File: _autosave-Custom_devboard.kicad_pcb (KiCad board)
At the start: 2 copper layers, 21 x 51 mm, 32 parts, among them J1 USB_C_Receptacle_USB2.0_14P, J2 Conn_01x20, J3 Conn_01x20, J4 Conn_01x03, SW1 SW_Push, U1 RP2040, U2 MCP1700x-330xxTT, U4 W25Q16JVZPIQ TR, Y1 12 MHz

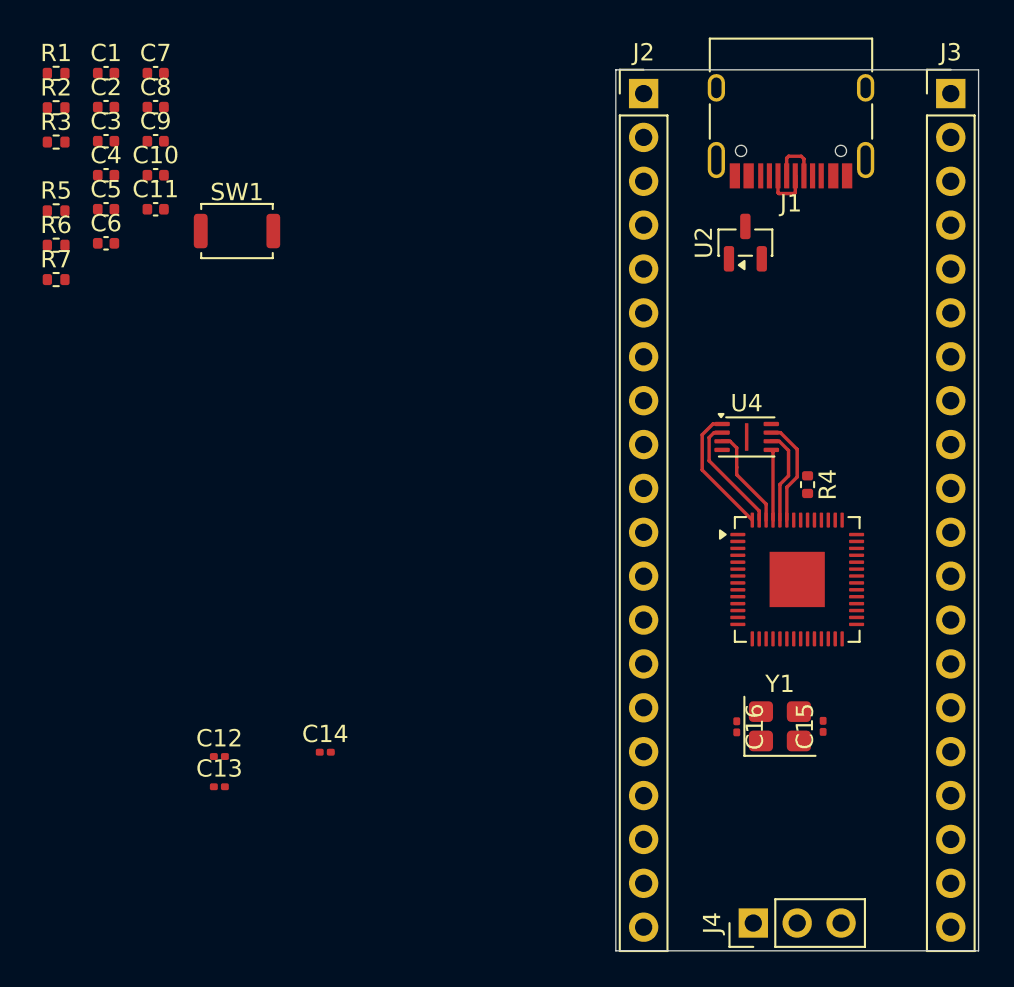
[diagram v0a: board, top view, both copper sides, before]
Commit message: PCB, CONECTING EVERYHTING SUCKS SO BAD
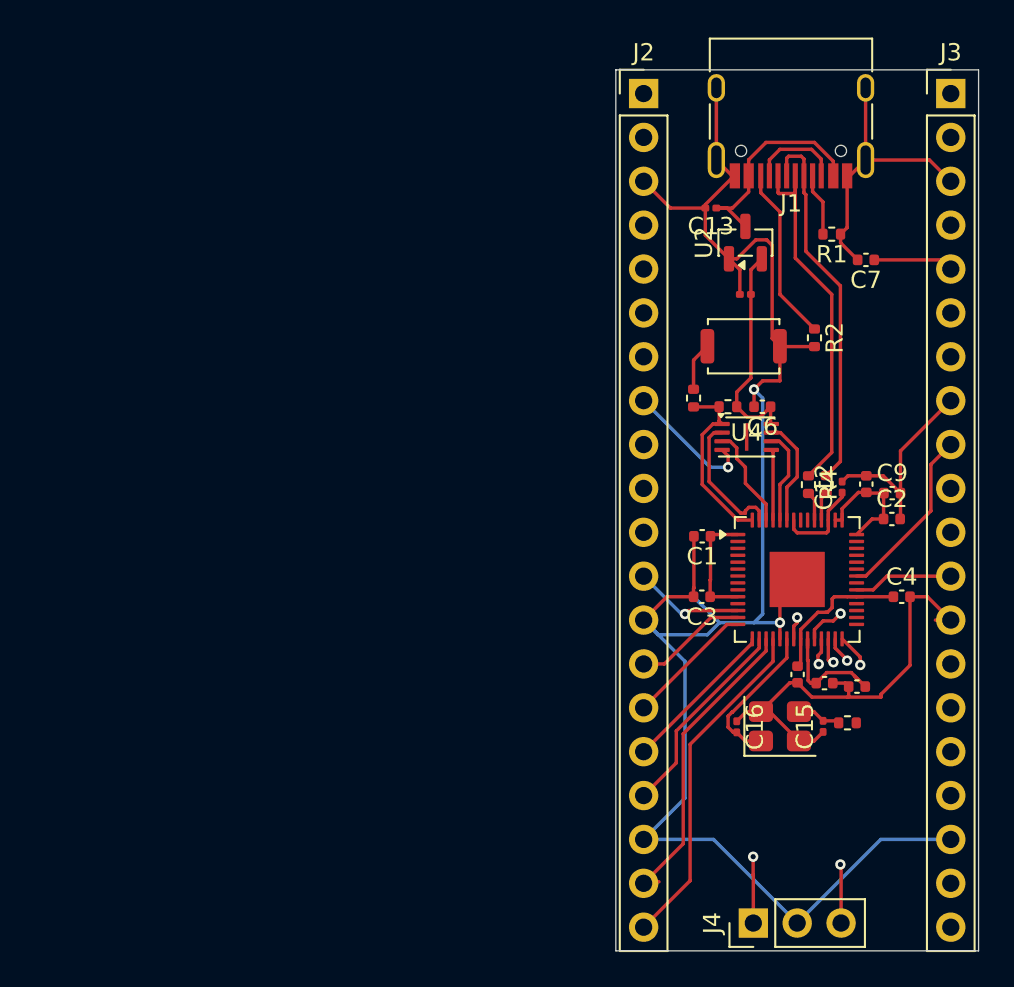
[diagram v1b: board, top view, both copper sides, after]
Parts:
- moved R5 54.6 mm to (216.4, 111.3)
- moved C4 52.1 mm to (219.6, 104.0)
- moved C2 51.4 mm to (219.0, 99.5)
- moved C10 50.2 mm to (217.0, 109.2), turned to 180 degrees
- moved R3 48.8 mm to (215.2, 97.5), turned to -90 degrees
- moved C5 48.2 mm to (213.5, 108.5), turned to -90 degrees
- moved C11 47.5 mm to (215.1, 109.0)
- moved C9 47.3 mm to (219.0, 98.0)
- moved C8 46.6 mm to (217.5, 97.5), turned to 90 degrees
- moved R2 45.9 mm to (214.5, 89.0), turned to -90 degrees
- moved R1 45.9 mm to (215.5, 83.0), turned to 180 degrees
- moved C13 44.0 mm to (208.5, 81.5), turned to 180 degrees
- moved C1 43.7 mm to (208.0, 100.5), turned to 180 degrees
- moved C3 43.4 mm to (208.0, 104.0), turned to 180 degrees
- moved C7 42.5 mm to (217.5, 84.5), turned to 180 degrees
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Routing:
- net GND: track 0.00 -> 169.0 mm, vias 0 -> 3
- net +3V3: track 0.00 -> 40.0 mm
- net GPIO15: track 0.00 -> 19.8 mm
- net USBD+: track 2.99 -> 21.8 mm
- net USBD-: track 3.11 -> 21.7 mm
- net GPIO14: track 0.00 -> 18.0 mm
- net VBUS: track 0.00 -> 13.0 mm
- net +1V1: track 0.00 -> 12.7 mm
- net GPIO13: track 0.00 -> 11.8 mm
- net GPIO24: track 0.00 -> 10.2 mm
- net Net-(J1-CC2): track 0.00 -> 10.2 mm
- net GPIO12: track 0.00 -> 9.14 mm
- net XIN: track 0.00 -> 8.77 mm
- net GPIO11: track 0.00 -> 7.45 mm
- net GPIO10: track 0.00 -> 6.57 mm
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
